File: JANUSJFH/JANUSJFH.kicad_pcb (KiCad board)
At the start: 2 copper layers, 30 parts, among them J1 USB_B_Micro, SW1 SW_SPDT, U1 STM32L476RGTx, U2 AMS1117-3.3, U3 BMP280, U4 IP4234CZ6

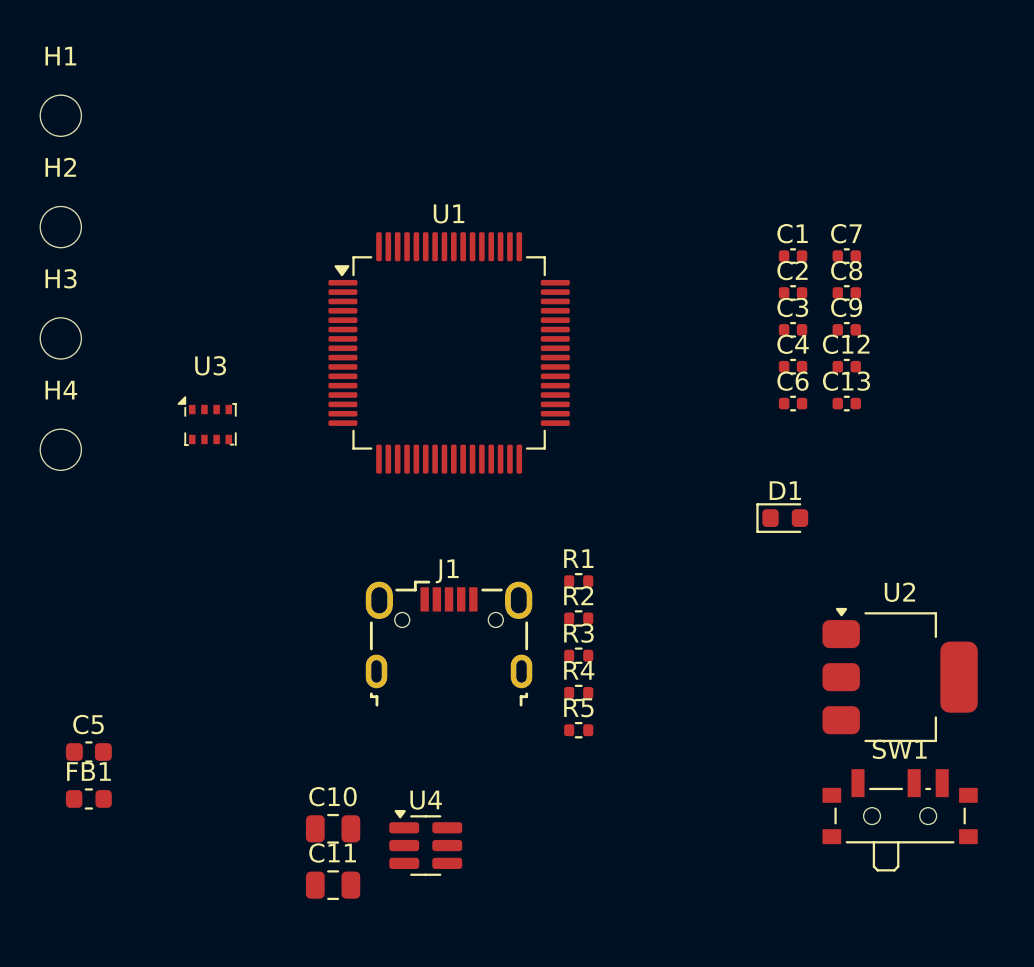
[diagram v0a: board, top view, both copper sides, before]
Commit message: Add files via upload
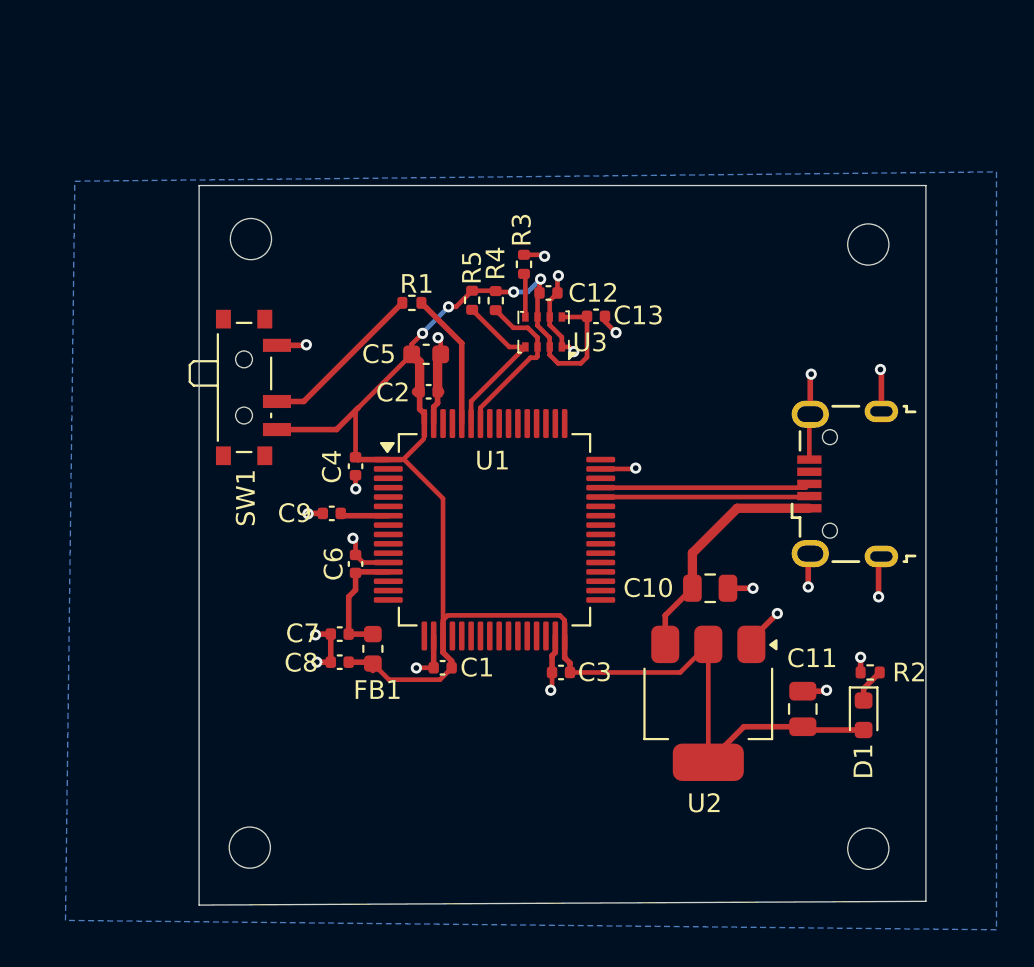
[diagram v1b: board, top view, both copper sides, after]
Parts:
- removed U4: IP4234CZ6, Package_TO_SOT_SMD:SC-74-6_1.55x2.9mm_P0.95mm
- moved H3 51.0 mm to (144.2, 95.7)
- moved H2 43.2 mm to (144.2, 63.4)
- moved SW1 41.4 mm to (111.1, 71.0), turned to -90 degrees
- moved H1 40.4 mm to (111.1, 95.6)
- moved C7 33.8 mm to (115.9, 84.2), turned to 180 degrees
- moved C8 33.5 mm to (115.9, 85.7), turned to 180 degrees
- moved C9 29.2 mm to (115.5, 77.8), turned to 180 degrees
- moved C1 28.9 mm to (121.4, 86.0), turned to 180 degrees
- moved C5 27.9 mm to (120.5, 69.2)
- moved C11 26.8 mm to (140.7, 88.2), turned to 90 degrees
- moved C6 24.9 mm to (116.8, 80.5), turned to 90 degrees
- moved C4 24.0 mm to (116.8, 75.2), turned to -90 degrees
- moved C10 23.9 mm to (135.7, 81.8)
- moved R5 23.7 mm to (123.0, 66.4), turned to 90 degrees
- moved J1 22.6 mm to (142.9, 76.2), turned to 90 degrees
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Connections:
- J1 pad 2: Net-(J1-D-) -> /USB_OTG_FS_DM-
- J1 pad 3: Net-(J1-D+) -> /USB_OTG_FS_DP+
- R4 pad 1: /I2C1_SCL -> /I2C1_SDA
- R5 pad 1: /I2C1_SDA -> /I2C1_SCL
- U1 pad 58: /I2C1_SCL -> /I2C1_SDA
- U1 pad 59: /I2C1_SDA -> /I2C1_SCL
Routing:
- net +3.3V: track 0.00 -> 92.6 mm, vias 0 -> 4
- net GND: track 0.00 -> 45.6 mm, vias 0 -> 22
- net VBUS: track 0.00 -> 12.7 mm
- net /USB_OTG_FS_DM-: track 0.00 -> 11.2 mm
- net /USB_OTG_FS_DP+: track 0.00 -> 11.2 mm
- net /I2C1_SCL: track 0.00 -> 9.00 mm
- net /SW_BOOT0: track 0.00 -> 8.88 mm
- net /I2C1_SDA: track 0.00 -> 8.88 mm
- net /BOOT0: track 0.00 -> 7.34 mm
- net +3.3VA: track 0.00 -> 6.48 mm
- net /NRST: track 0.00 -> 2.59 mm
- net Net-(U3-SDO): track 0.00 -> 2.36 mm
- net Net-(D1-K): track 0.00 -> 1.86 mm
- added copper zone on B.Cu, net GND
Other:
- board outline added: 38.8 x 38.5 mm
